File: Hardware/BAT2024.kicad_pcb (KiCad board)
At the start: 2 copper layers, 80 x 80 mm, 55 parts, among them IC1 BGM220PC22WGA2R, IC2 EEPROM_M95P16-IXMNT_E, IC3 LED-Driver_LP55231SQX_NOPB, J1 Conn_ARM_SWD_TagConnect_TC203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, J2 USB4105-GF-A-060, U1 MIC5504-3.3YM5, U2 BQ21040DBVR

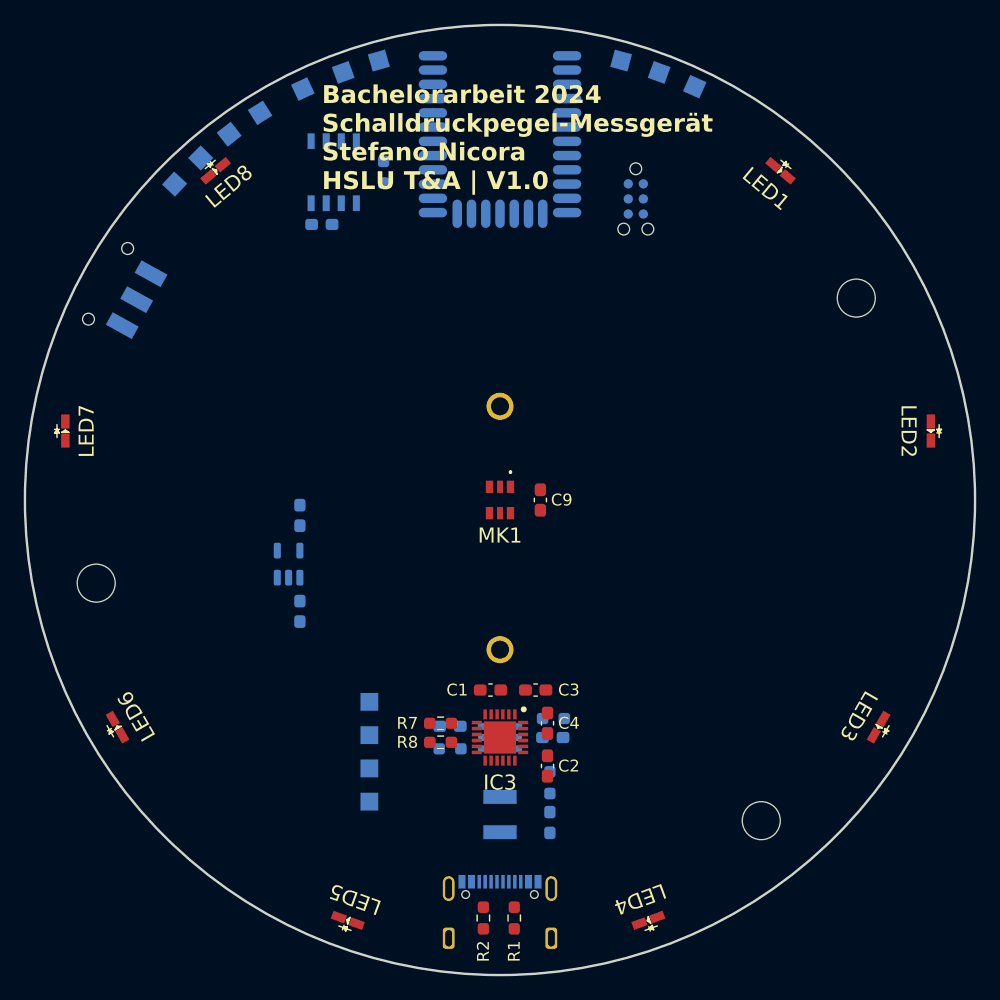
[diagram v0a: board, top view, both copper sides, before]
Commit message: Created first layout
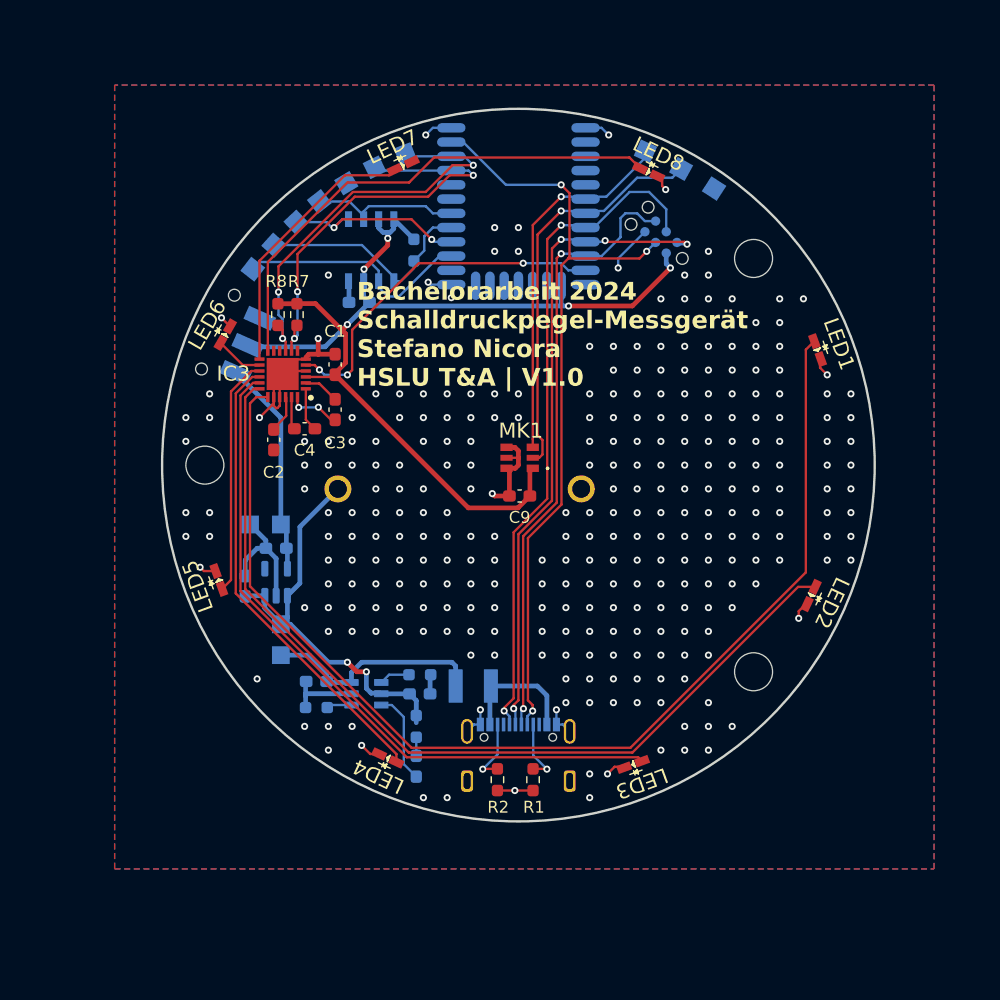
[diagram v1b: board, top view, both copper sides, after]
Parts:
- moved R8 38.5 mm to (94.0, 44.7), turned to -90 degrees
- moved R7 36.5 mm to (95.6, 44.7), turned to -90 degrees
- moved LED8 36.5 mm to (125.2, 32.7), turned to 155 degrees
- moved LED7 36.2 mm to (104.5, 32.1), turned to -155 degrees
- moved C2 35.9 mm to (93.6, 55.2)
- moved IC3 35.7 mm to (94.4, 49.7), turned to 180 degrees
- moved LED6 34.3 mm to (89.5, 46.3), turned to -120 degrees
- moved C4 32.1 mm to (96.2, 54.3), turned to 180 degrees
- moved LED5 30.6 mm to (89.0, 67.0), turned to -70 degrees
- moved C1 30.4 mm to (98.8, 48.9), turned to 90 degrees
- moved C3 29.0 mm to (98.8, 52.7), turned to -90 degrees
- moved LED4 25.9 mm to (103.2, 82.0), turned to -25 degrees
- moved TP6 22.9 mm to (91.6, 62.3)
- moved LED3 20.9 mm to (123.9, 82.5), turned to 20 degrees
- moved LED2 17.1 mm to (138.9, 68.3), turned to 65 degrees
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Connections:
- net Net-(F1-Pad1) renamed Fuse
- C8 pad 1: +3.3V -> +3.3
- J1 pad 1: VCC -> +3.3V
- J2 pad A7: /RESET -> /SWDIO
- J2 pad B7: /SWDIO -> /RESET
- S1 pad 1: Net-(U1-VOUT) -> +3.3
- TP3 pad 1: +3.3V -> +3.3
- U1 pad 5: Net-(U1-VOUT) -> +3.3
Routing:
- net /LED1: track 0.00 -> 95.4 mm
- net +3.3V: track 0.00 -> 92.0 mm, vias 0 -> 5
- net /LED2: track 0.00 -> 77.1 mm
- net GND: track 0.00 -> 75.2 mm, vias 0 -> 294
- net /RESET: track 0.00 -> 66.2 mm, vias 0 -> 3
- net /LED3: track 0.00 -> 58.3 mm
- net /SWCLK: track 0.00 -> 56.7 mm, vias 0 -> 2
- net /SWDIO: track 0.00 -> 54.3 mm, vias 0 -> 4
- net /SWO: track 0.00 -> 51.8 mm, vias 0 -> 2
- net /LED8: track 0.00 -> 42.8 mm
- net /LED4: track 0.00 -> 39.2 mm
- net /I2C_SDA: track 0.00 -> 35.1 mm, vias 0 -> 3
- net +BATT: track 0.00 -> 34.8 mm, vias 0 -> 2
- net /I2C_SCL: track 0.00 -> 34.7 mm, vias 0 -> 3
- net /PDM_CLK: track 0.00 -> 34.0 mm, vias 0 -> 1
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- added copper zone on B.Cu, net GND
- added copper zone on F.Cu, net GND
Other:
- board size 80 x 80 mm -> 60 x 60 mm
- board text added: "CS"
- board text added: "DATA0"
- board text added: "MISO"
- board text added: "MOSI"
- board text added: "SCK"
- board text added: "SCL"
- board text added: "SDA"
